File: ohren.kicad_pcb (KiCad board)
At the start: 2 copper layers, 100 x 100 mm, 42 parts, among them J1 Conn_01x19_MountingPin, U1 TLC5955RTQ

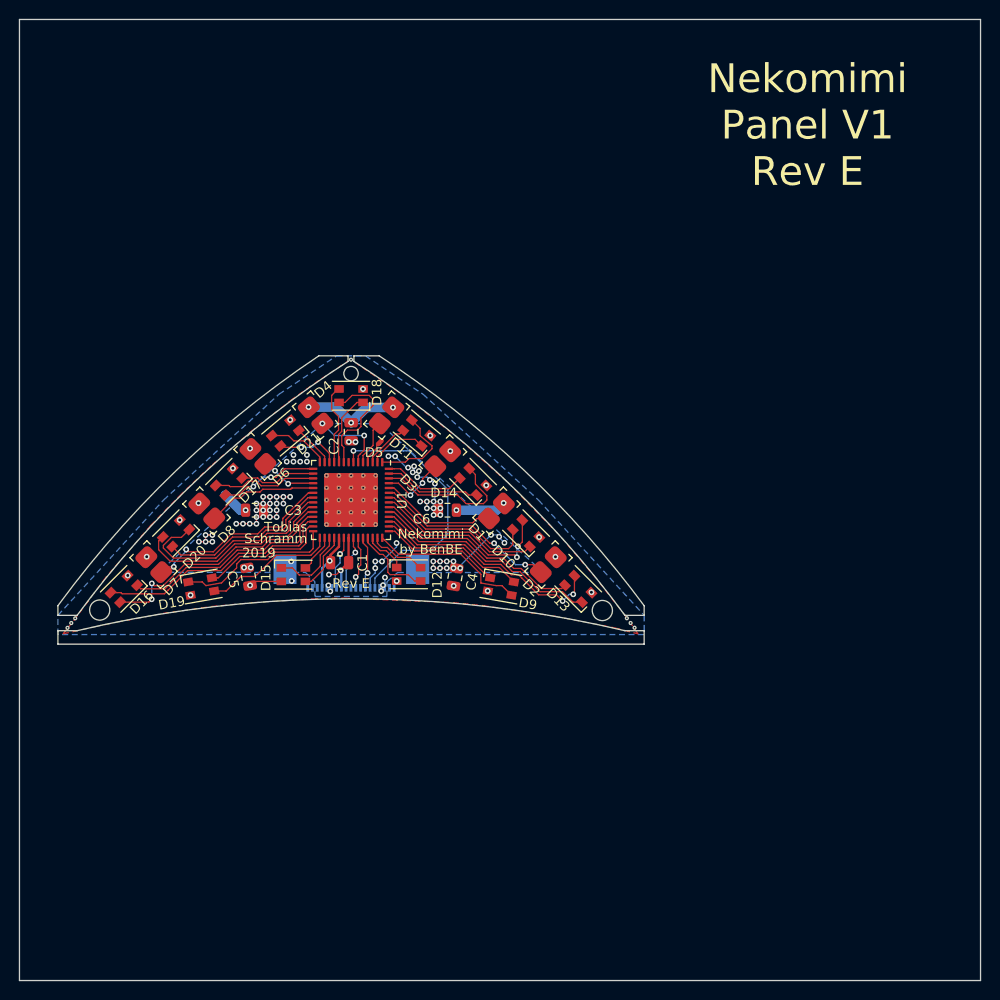
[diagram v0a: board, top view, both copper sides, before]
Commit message: Finish panel
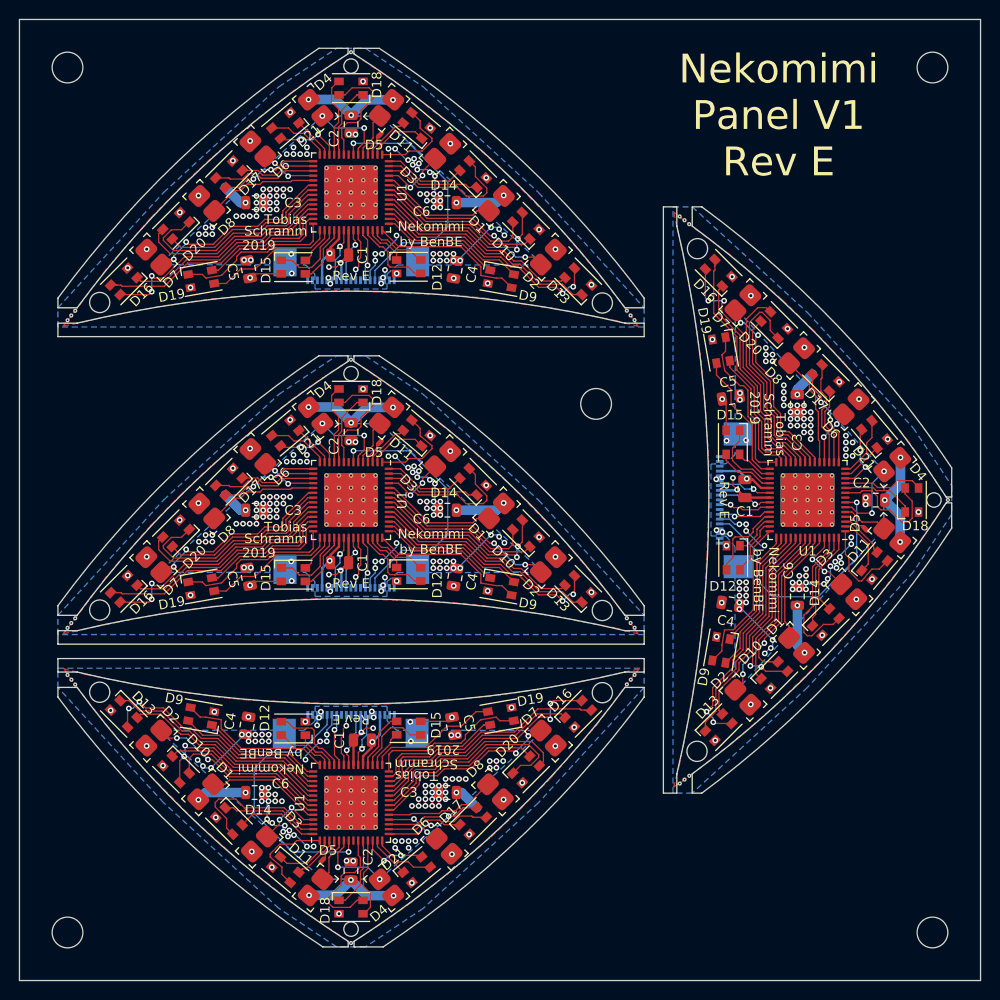
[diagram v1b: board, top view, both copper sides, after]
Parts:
- added C1: C, Capacitor_SMD:C_0805_2012Metric, F.Cu at (175.5, 148.8)
- added C1: C, Capacitor_SMD:C_0805_2012Metric, F.Cu at (135.7, 175.0)
- added C1: C, Capacitor_SMD:C_0805_2012Metric, F.Cu at (133.3, 124.5)
- added C2: C, Capacitor_SMD:C_0805_2012Metric, F.Cu at (189.1, 150.0)
- added C2: C, Capacitor_SMD:C_0805_2012Metric, F.Cu at (134.5, 188.6)
- added C2: C, Capacitor_SMD:C_0805_2012Metric, F.Cu at (134.5, 110.9)
- added C3: C, Capacitor_SMD:C_0805_2012Metric, F.Cu at (180.9, 140.0)
- added C3: C, Capacitor_SMD:C_0805_2012Metric, F.Cu at (144.5, 180.4)
- added C3: C, Capacitor_SMD:C_0805_2012Metric, F.Cu at (124.5, 119.1)
- added C4: C, Capacitor_SMD:C_0805_2012Metric, F.Cu at (174.0, 160.8)
- added C4: C, Capacitor_SMD:C_0805_2012Metric, F.Cu at (123.7, 173.5)
- added C4: C, Capacitor_SMD:C_0805_2012Metric, F.Cu at (145.3, 126.0)
- added C5: C, Capacitor_SMD:C_0805_2012Metric, F.Cu at (174.0, 139.3)
- added C5: C, Capacitor_SMD:C_0805_2012Metric, F.Cu at (145.2, 173.5)
- added C5: C, Capacitor_SMD:C_0805_2012Metric, F.Cu at (123.8, 126.0)
- added C6: C, Capacitor_SMD:C_0805_2012Metric, F.Cu at (180.9, 160.0)
- added C6: C, Capacitor_SMD:C_0805_2012Metric, F.Cu at (124.5, 180.4)
- added C6: C, Capacitor_SMD:C_0805_2012Metric, F.Cu at (144.5, 119.1)
- added D1: LED, catear-pcb:smd_led_universal, F.Cu at (180.9, 165.1)
- added D1: LED, catear-pcb:smd_led_universal, F.Cu at (119.4, 180.4)
- added D1: LED, catear-pcb:smd_led_universal, F.Cu at (149.6, 119.1)
- added D10: LED_ARGB, catear-pcb:ASMB-MTB1-0A3A2, F.Cu at (178.5, 168.2)
- added D10: LED_ARGB, catear-pcb:ASMB-MTB1-0A3A2, F.Cu at (116.3, 178.0)
- added D10: LED_ARGB, catear-pcb:ASMB-MTB1-0A3A2, F.Cu at (152.7, 121.5)
- added D11: LED_ARGB, catear-pcb:ASMB-MTB1-0A3A2, F.Cu at (189.0, 156.8)
- added D11: LED_ARGB, catear-pcb:ASMB-MTB1-0A3A2, F.Cu at (127.7, 188.5)
- added D11: LED_ARGB, catear-pcb:ASMB-MTB1-0A3A2, F.Cu at (141.3, 111.0)
- added D12: LED_ARGB, catear-pcb:ASMB-MTB1-0A3A2, F.Cu at (174.3, 156.0)
- added D12: LED_ARGB, catear-pcb:ASMB-MTB1-0A3A2, F.Cu at (128.5, 173.8)
- added D12: LED_ARGB, catear-pcb:ASMB-MTB1-0A3A2, F.Cu at (140.5, 125.7)
- added D13: LED_ARGB, catear-pcb:ASMB-MTB1-0A3A2, F.Cu at (172.8, 173.6)
- added D13: LED_ARGB, catear-pcb:ASMB-MTB1-0A3A2, F.Cu at (110.9, 172.2)
- added D13: LED_ARGB, catear-pcb:ASMB-MTB1-0A3A2, F.Cu at (158.1, 127.2)
- added D14: LED_ARGB, catear-pcb:ASMB-MTB1-0A3A2, F.Cu at (183.9, 162.7)
- added D14: LED_ARGB, catear-pcb:ASMB-MTB1-0A3A2, F.Cu at (121.8, 183.4)
- added D14: LED_ARGB, catear-pcb:ASMB-MTB1-0A3A2, F.Cu at (147.2, 116.1)
- added D15: LED_ARGB, catear-pcb:ASMB-MTB1-0A3A2, F.Cu at (174.2, 144.0)
- added D15: LED_ARGB, catear-pcb:ASMB-MTB1-0A3A2, F.Cu at (140.5, 173.7)
- added D15: LED_ARGB, catear-pcb:ASMB-MTB1-0A3A2, F.Cu at (128.5, 125.8)
- added D16: LED_ARGB, catear-pcb:ASMB-MTB1-0A3A2, F.Cu at (172.8, 126.4)
- added D16: LED_ARGB, catear-pcb:ASMB-MTB1-0A3A2, F.Cu at (158.1, 172.2)
- added D16: LED_ARGB, catear-pcb:ASMB-MTB1-0A3A2, F.Cu at (110.9, 127.2)
- added D17: LED_ARGB, catear-pcb:ASMB-MTB1-0A3A2, F.Cu at (183.9, 137.3)
- added D17: LED_ARGB, catear-pcb:ASMB-MTB1-0A3A2, F.Cu at (147.2, 183.4)
- added D17: LED_ARGB, catear-pcb:ASMB-MTB1-0A3A2, F.Cu at (121.8, 116.1)
- added D18: LED_ARGB, catear-pcb:ASMB-MTB1-0A3A2, F.Cu at (192.8, 150.0)
- added D18: LED_ARGB, catear-pcb:ASMB-MTB1-0A3A2, F.Cu at (134.5, 192.3)
- added D18: LED_ARGB, catear-pcb:ASMB-MTB1-0A3A2, F.Cu at (134.5, 107.2)
- added D19: LED_ARGB, catear-pcb:ASMB-MTB1-0A3A2, F.Cu at (173.0, 134.4)
- added D19: LED_ARGB, catear-pcb:ASMB-MTB1-0A3A2, F.Cu at (150.1, 172.5)
- added D19: LED_ARGB, catear-pcb:ASMB-MTB1-0A3A2, F.Cu at (118.9, 127.0)
- added D2: LED, catear-pcb:smd_led_universal, F.Cu at (175.3, 170.5)
- added D2: LED, catear-pcb:smd_led_universal, F.Cu at (114.0, 174.8)
- added D2: LED, catear-pcb:smd_led_universal, F.Cu at (155.0, 124.7)
- added D20: LED_ARGB, catear-pcb:ASMB-MTB1-0A3A2, F.Cu at (178.5, 131.8)
- added D20: LED_ARGB, catear-pcb:ASMB-MTB1-0A3A2, F.Cu at (152.7, 178.0)
- added D20: LED_ARGB, catear-pcb:ASMB-MTB1-0A3A2, F.Cu at (116.3, 121.5)
- added D21: LED_ARGB, catear-pcb:ASMB-MTB1-0A3A2, F.Cu at (189.0, 143.2)
- added D21: LED_ARGB, catear-pcb:ASMB-MTB1-0A3A2, F.Cu at (141.3, 188.5)
- added D21: LED_ARGB, catear-pcb:ASMB-MTB1-0A3A2, F.Cu at (127.7, 111.0)
- added D3: LED, catear-pcb:smd_led_universal, F.Cu at (186.3, 159.6)
- added D3: LED, catear-pcb:smd_led_universal, F.Cu at (124.9, 185.8)
- added D3: LED, catear-pcb:smd_led_universal, F.Cu at (144.1, 113.7)
- added D4: LED, catear-pcb:smd_led_universal, F.Cu at (190.8, 146.3)
- added D4: LED, catear-pcb:smd_led_universal, F.Cu at (138.2, 190.3)
- added D4: LED, catear-pcb:smd_led_universal, F.Cu at (130.8, 109.2)
- added D5: LED, catear-pcb:smd_led_universal, F.Cu at (190.8, 153.7)
- added D5: LED, catear-pcb:smd_led_universal, F.Cu at (130.8, 190.3)
- added D5: LED, catear-pcb:smd_led_universal, F.Cu at (138.2, 109.2)
- added D6: LED, catear-pcb:smd_led_universal, F.Cu at (186.6, 140.3)
- added D6: LED, catear-pcb:smd_led_universal, F.Cu at (144.2, 186.1)
- added D6: LED, catear-pcb:smd_led_universal, F.Cu at (124.8, 113.5)
- added D7: LED, catear-pcb:smd_led_universal, F.Cu at (175.3, 129.5)
- added D7: LED, catear-pcb:smd_led_universal, F.Cu at (155.0, 174.8)
- added D7: LED, catear-pcb:smd_led_universal, F.Cu at (114.0, 124.7)
- added D8: LED, catear-pcb:smd_led_universal, F.Cu at (180.9, 135.0)
- added D8: LED, catear-pcb:smd_led_universal, F.Cu at (149.5, 180.4)
- added D8: LED, catear-pcb:smd_led_universal, F.Cu at (119.5, 119.1)
- added D9: LED_ARGB, catear-pcb:ASMB-MTB1-0A3A2, F.Cu at (173.0, 165.6)
- added D9: LED_ARGB, catear-pcb:ASMB-MTB1-0A3A2, F.Cu at (118.9, 172.5)
- added D9: LED_ARGB, catear-pcb:ASMB-MTB1-0A3A2, F.Cu at (150.1, 127.0)
- added G***: LOGO, catear-pcb:attribution, B.Cu at (173.0, 132.5)
- added G***: LOGO, catear-pcb:catboy, B.Cu at (177.0, 165.0)
- added G***: LOGO, catear-pcb:attribution, B.Cu at (152.0, 172.5)
- added G***: LOGO, catear-pcb:catboy, B.Cu at (119.5, 176.5)
- added G***: LOGO, catear-pcb:attribution, B.Cu at (117.0, 127.0)
- added G***: LOGO, catear-pcb:catboy, B.Cu at (149.5, 123.0)
- added J1: Conn_01x19_MountingPin, catear-pcb:Molex_Easy-On_52746-1971_1x19_P0.5mm_Horizontal, B.Cu at (172.9, 150.0)
- added J1: Conn_01x19_MountingPin, catear-pcb:Molex_Easy-On_52746-1971_1x19_P0.5mm_Horizontal, B.Cu at (134.5, 172.4)
- added J1: Conn_01x19_MountingPin, catear-pcb:Molex_Easy-On_52746-1971_1x19_P0.5mm_Horizontal, B.Cu at (134.5, 127.1)
- added REF**: MountingHole_3.2mm_M3, MountingHole:MountingHole_3.2mm_M3, F.Cu at (160.0, 140.0)
- added REF**: npth_0.3, catear-pcb:npth_0.3, F.Cu at (169.2, 179.1)
- added REF**: npth_0.3, catear-pcb:npth_0.3, F.Cu at (168.7, 179.5)
- added REF**: npth_0.3, catear-pcb:npth_0.3, B.Cu at (169.7, 121.3)
- added REF**: MountingHole_2.1mm, MountingHole:MountingHole_2.1mm, F.Cu at (170.6, 123.8)
- added REF**: MountingHole_1.5mm, catear-pcb:MountingHole_1mm, F.Cu at (195.2, 150.0)
- added REF**: MountingHole_2.1mm, MountingHole:MountingHole_2.1mm, F.Cu at (170.5, 176.2)
- added REF**: npth_0.3, catear-pcb:npth_0.3, F.Cu at (134.5, 196.1)
- added REF**: npth_0.3, catear-pcb:npth_0.3, B.Cu at (164.0, 168.2)
- added REF**: npth_0.3, catear-pcb:npth_0.3, B.Cu at (163.6, 168.7)
- added REF**: npth_0.3, catear-pcb:npth_0.3, F.Cu at (105.8, 169.2)
- added REF**: MountingHole_3.2mm_M3, MountingHole:MountingHole_3.2mm_M3, F.Cu at (195.0, 195.0)
- added REF**: npth_0.3, catear-pcb:npth_0.3, F.Cu at (105.4, 168.7)
- added REF**: npth_0.3, catear-pcb:npth_0.3, F.Cu at (105.0, 168.2)
- added REF**: npth_0.3, catear-pcb:npth_0.3, B.Cu at (163.2, 169.2)
- added REF**: MountingHole_2.1mm, MountingHole:MountingHole_2.1mm, F.Cu at (160.7, 170.1)
- added REF**: MountingHole_1.5mm, catear-pcb:MountingHole_1mm, F.Cu at (134.5, 194.7)
- added REF**: MountingHole_2.1mm, MountingHole:MountingHole_2.1mm, F.Cu at (108.3, 170.0)
- added REF**: npth_0.3, catear-pcb:npth_0.3, F.Cu at (134.5, 103.4)
- added REF**: npth_0.3, catear-pcb:npth_0.3, B.Cu at (105.0, 131.3)
- added REF**: npth_0.3, catear-pcb:npth_0.3, B.Cu at (105.4, 130.8)
- added REF**: npth_0.3, catear-pcb:npth_0.3, F.Cu at (163.2, 130.3)
- added REF**: MountingHole_3.2mm_M3, MountingHole:MountingHole_3.2mm_M3, F.Cu at (105.0, 195.0)
- added REF**: npth_0.3, catear-pcb:npth_0.3, F.Cu at (163.6, 130.8)
- added REF**: npth_0.3, catear-pcb:npth_0.3, F.Cu at (164.0, 131.3)
- added REF**: npth_0.3, catear-pcb:npth_0.3, B.Cu at (105.8, 130.3)
- added REF**: MountingHole_2.1mm, MountingHole:MountingHole_2.1mm, F.Cu at (108.3, 129.4)
- added REF**: MountingHole_1.5mm, catear-pcb:MountingHole_1mm, F.Cu at (134.5, 104.8)
- added REF**: MountingHole_2.1mm, MountingHole:MountingHole_2.1mm, F.Cu at (160.7, 129.5)
- added REF**: MountingHole_3.2mm_M3, MountingHole:MountingHole_3.2mm_M3, F.Cu at (105.0, 105.0)
- added REF**: MountingHole_3.2mm_M3, MountingHole:MountingHole_3.2mm_M3, F.Cu at (195.0, 105.0)
- added REF**: npth_0.3, catear-pcb:npth_0.3, F.Cu at (196.6, 150.0)
- added REF**: npth_0.3, catear-pcb:npth_0.3, B.Cu at (168.7, 120.5)
- added REF**: npth_0.3, catear-pcb:npth_0.3, B.Cu at (169.2, 120.9)
- added REF**: npth_0.3, catear-pcb:npth_0.3, F.Cu at (169.7, 178.7)
- added TP1: TestPoint, catear-pcb:TestPoint_0.5x1mm, F.Cu at (188.0, 153.0)
- added TP1: TestPoint, catear-pcb:TestPoint_0.5x1mm, F.Cu at (131.5, 187.5)
- added TP1: TestPoint, catear-pcb:TestPoint_0.5x1mm, F.Cu at (137.5, 112.0)
- added U1: TLC5955RTQ, Package_DFN_QFN:QFN-56-1EP_8x8mm_P0.5mm_EP5.6x5.6mm_ThermalVias, F.Cu at (182.0, 150.0)
- added U1: TLC5955RTQ, Package_DFN_QFN:QFN-56-1EP_8x8mm_P0.5mm_EP5.6x5.6mm_ThermalVias, F.Cu at (134.5, 181.5)
- added U1: TLC5955RTQ, Package_DFN_QFN:QFN-56-1EP_8x8mm_P0.5mm_EP5.6x5.6mm_ThermalVias, F.Cu at (134.5, 118.0)
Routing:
- net (no net): track 0.00 -> 2235.2 mm, vias 0 -> 393
- added copper zone on B.Cu, net (none)
- added copper zone on F.Cu, net (none)
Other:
- outline, holes or cut-outs redrawn
